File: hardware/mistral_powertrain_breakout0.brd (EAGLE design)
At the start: 37.3 x 41.1 mm, 24 parts, among them U1 MCP73831, U2 MCP73833-GPI/UN

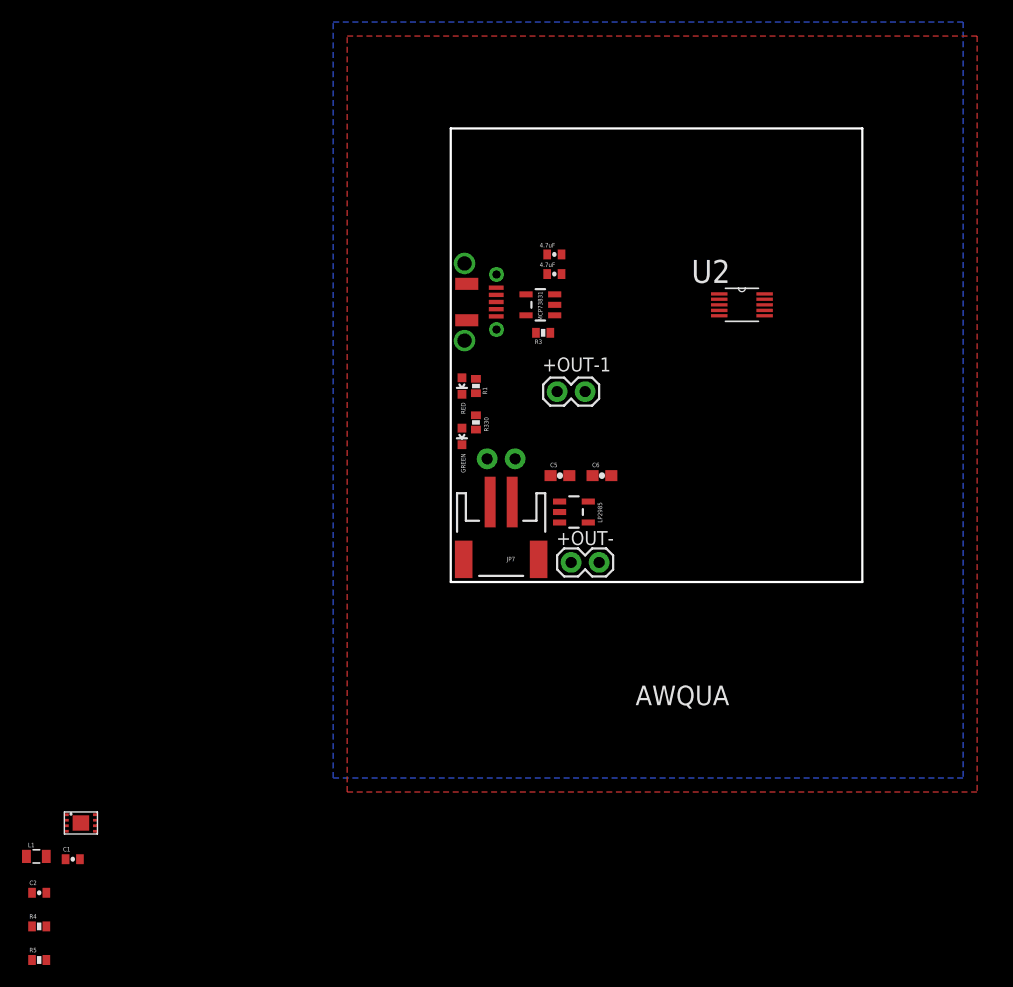
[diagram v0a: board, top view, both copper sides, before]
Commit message: board updates
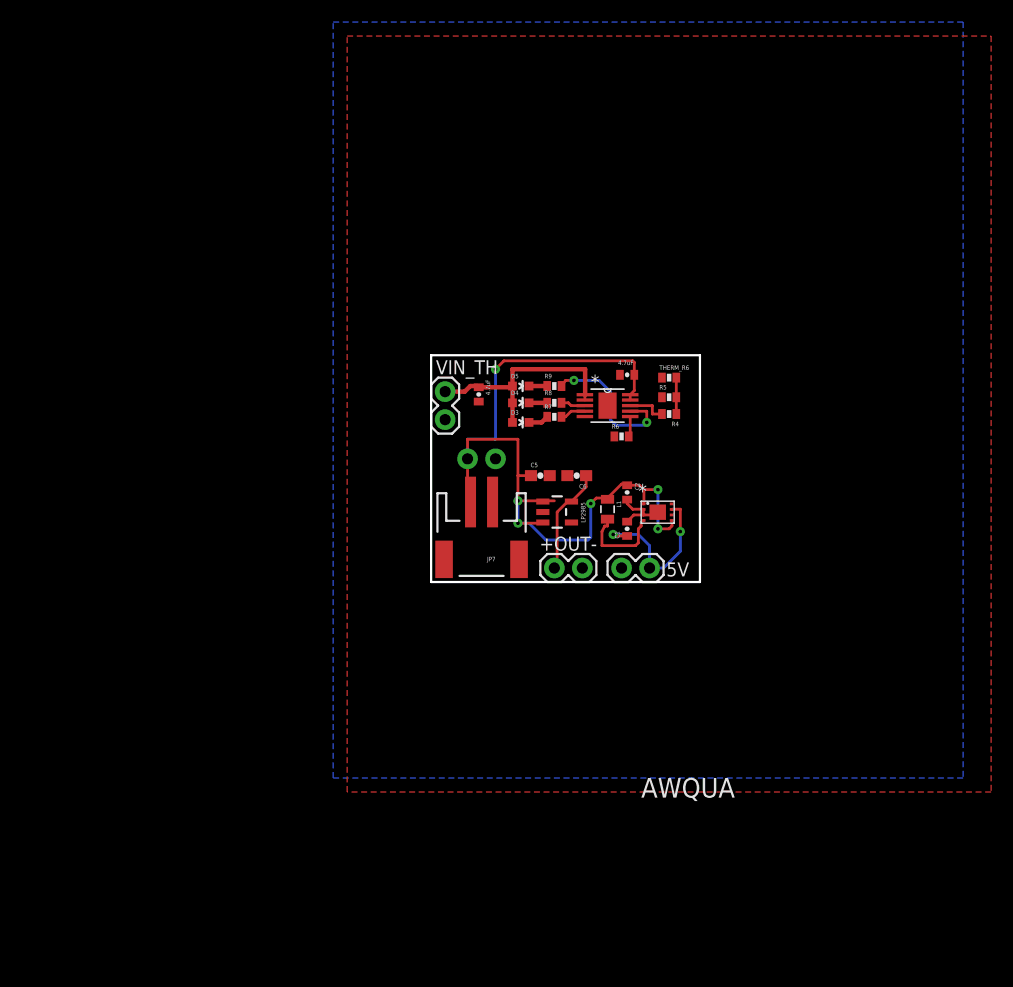
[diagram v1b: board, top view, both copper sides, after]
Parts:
- removed +OUT-1: (no value), SparkFun-Connectors:1X02
- removed D1: RED, SparkFun:LED-0603
- removed D2: GREEN, SparkFun:LED-0603
- removed R1, R2: R330, SparkFun:0402-RES
- removed R3: R2K, SparkFun:0402-RES
- removed U$3: USBMICRO-DX4R005JJ2, awqua_eagle_library:USBMICRO-DX4R005JJ2
- removed U1: MCP73831, SparkFun:SOT23-5
- added D3: BLUE, SparkFun:LED-0603
- added D4: GREEN, SparkFun:LED-0603
- added D5: RED, SparkFun:LED-0603
- added JMP1: (no value), SparkFun:1X02
- added R6: 1k, SparkFun:0402-RES
- added R7, R8, R9: R330, SparkFun:0402-RES
- added THERM_R6: 10k, SparkFun:0402-RES
- added VIN_TH: (no value), SparkFun-Connectors:1X02
- C5: value (none) -> 1uF
- R4: value R330 -> 1.54k
- R5: value R330 -> 69.8k
- U2: value MCP73833-GPI/UN -> MCP73833
- moved R5 76.6 mm to (21.6, 16.8)
- moved R4 73.7 mm to (21.6, 15.2), turned to 180 degrees
- moved C2 64.5 mm to (17.8, 8.13), turned to 270 degrees
- moved L1 60.6 mm to (16.0, 6.60), turned to 270 degrees
- moved U$1 59.4 mm to (19.1, 5.33)
- moved C1 58.5 mm to (17.8, 4.83), turned to 90 degrees
- moved U2 15.2 mm to (16.0, 16.0)
- moved C3 14.4 mm to (4.32, 17.0), turned to 270 degrees
- moved C4 11.3 mm to (17.8, 18.8), turned to 180 degrees
- moved C6 2.29 mm to (13.2, 9.65), turned to 180 degrees
- moved JMP 1.78 mm to (5.84, 11.2)
- moved JP7 1.78 mm to (4.57, 3.56)
- moved C5 1.78 mm to (9.91, 9.65)
- moved +OUT- 1.61 mm to (11.2, 1.27)
- moved U$2 1.52 mm to (10.2, 7.62)
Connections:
- removed net N$1: U2.1, U2.2
- removed net N$2: D2.A, R2.2
- removed net N$3: D1.A, R1.1
- removed net N$6: U2.5
- removed net PROG: R3.1, U1.5
- removed net STAT: D1.C, R2.1, U1.1
- new net N$10: R7.2, U2.4
- new net N$11: D3.C, R7.1
- new net N$12: R8.2, U2.3
- new net N$13: D4.C, R8.1
- new net N$15: D5.C, R9.1
- new net N$16: R9.2, U2.7
- new net N$7: R4.2, U2.8
- new net N$8: R4.1, R5.2, THERM_R6.2
- new net N$9: R6.2, U2.6
- net GND: now also JMP1.1, R5.1, R6.1, THERM_R6.1, U2.5, U2.P$1, VIN_TH.1; no longer +OUT-1.1, D2.C, R3.2, U$3.GND, U$3.HOLE0, U$3.HOLE1, U$3.HOLE2, U$3.HOLE3, U$3.PAD0, U$3.PAD1, U1.2
- net VBAT: now also U2.10, U2.9; no longer U1.3
- net VBOOST: now also JMP1.2
- net VIN: now also D3.A, D4.A, D5.A, U2.1, U2.2, VIN_TH.2; no longer +OUT-1.2, R1.2, U$3.VCC, U1.4
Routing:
- net VBAT: track 0.00 -> 76.5 mm, vias 0 -> 6
- net VIN: track 0.00 -> 21.2 mm
- net VBOOST: track 0.00 -> 15.0 mm, vias 0 -> 2
- net N$16: track 0.00 -> 13.9 mm, vias 0 -> 2
- net VCC: track 0.00 -> 9.78 mm
- net N$5: track 0.00 -> 8.34 mm
- net N$4: track 0.00 -> 5.68 mm
- net N$7: track 0.00 -> 3.64 mm
- net N$8: track 0.00 -> 3.30 mm
- net N$10: track 0.00 -> 2.33 mm
- net N$12: track 0.00 -> 2.22 mm
- net N$11: track 0.00 -> 1.86 mm
- net N$9: track 0.00 -> 1.83 mm
- net N$15: track 0.00 -> 1.65 mm
- net N$13: track 0.00 -> 1.65 mm
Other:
- board size 37.3 x 41.1 mm -> 24.4 x 20.6 mm
- board text added: "*"
- board text added: "5V"
- board text added: "Troposphere Mistral v0 Powertrain 2018-06-08 cdk"
- board text removed: "awqua power supply v2.0 2016/02/22 github.com/awqua"
